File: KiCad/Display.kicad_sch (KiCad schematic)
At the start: 30 parts, among them J1 DC, J2 USB-C, M1 OLED1.5-RGB, U1 L86-M33, U2 ESP32-PICO-MINI-02, U3 FT231XQ, U4 LMR16006+FB, U5 QR

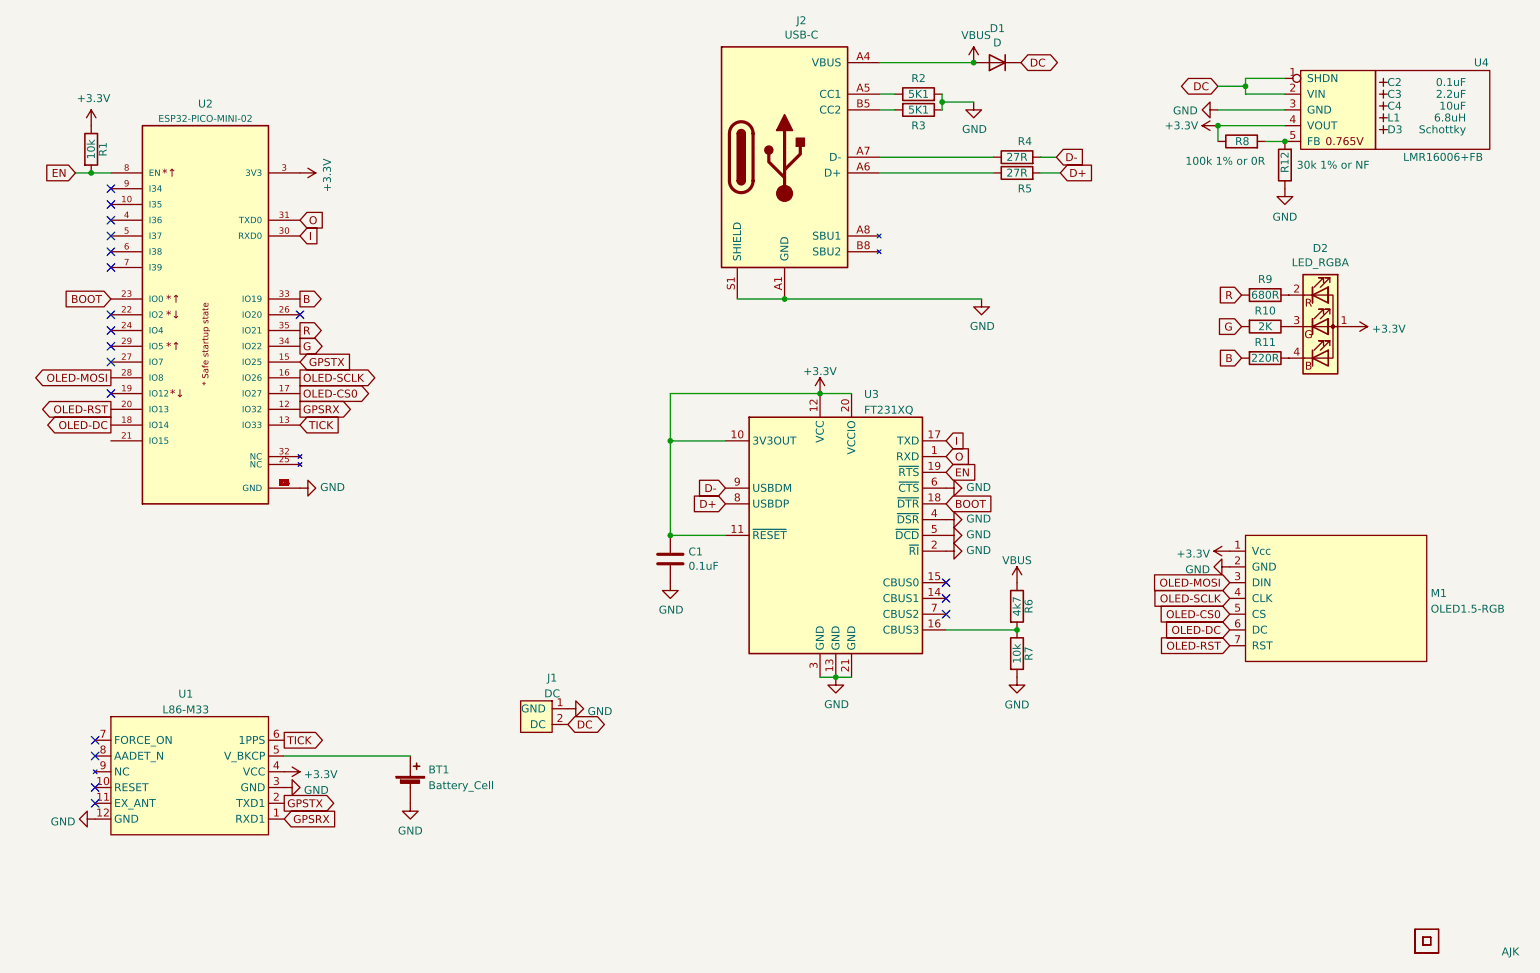
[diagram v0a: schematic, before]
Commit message: Pin names
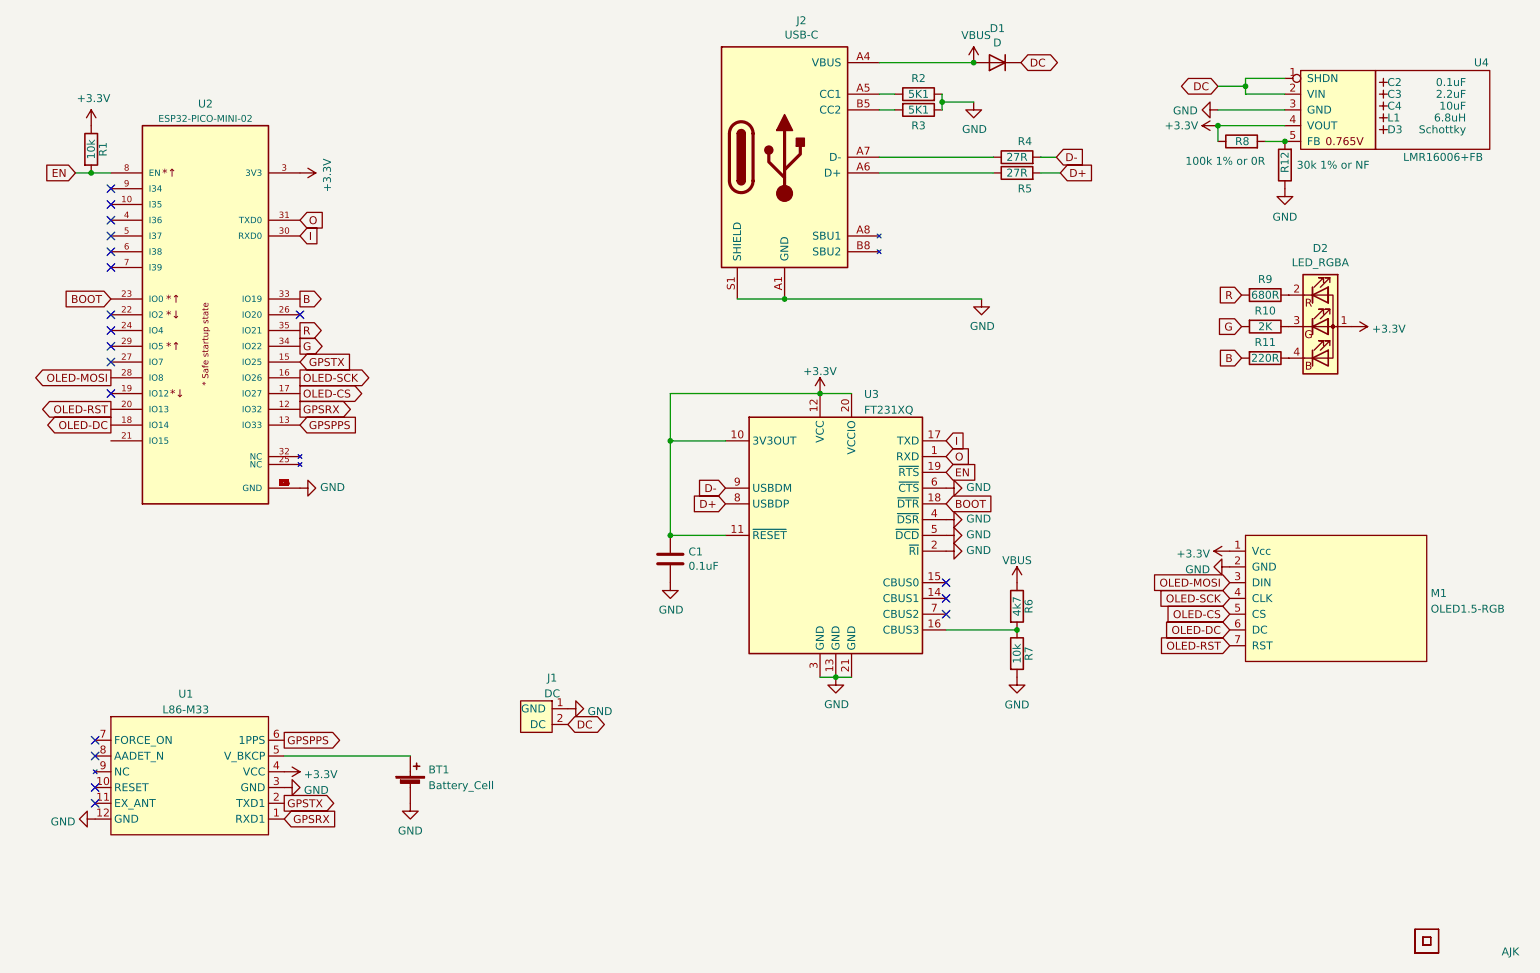
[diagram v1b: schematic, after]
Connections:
- net OLED-CS0 renamed OLED-CS
- net OLED-SCLK renamed OLED-SCK
- net TICK renamed GPSPPS
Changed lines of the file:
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@@
     )
   )
-  (global_label "OLED-SCLK" (shape input) (at 231.14 116.84 180) (fields_autoplaced)
+  (global_label "OLED-SCK" (shape input) (at 231.14 116.84 180) (fields_autoplaced)
     (effects (font (size 1.27 1.27)) (justify right))
-    (property "Intersheet References" "${INTERSHEET_REFS}" (id 0) (at 121.285 -13.335 0)
-      (effects (font (size 1.27 1.27)) hide)
+    (property "Intersheet References" "${INTERSHEET_REFS}" (id 0) (at 218.7163 116.7606 0)
+      (effects (font (size 1.27 1.27)) (justify right) hide)
     )
   )
@@
     )
   )
-  (global_label "OLED-CS0" (shape input) (at 231.14 119.38 180) (fields_autoplaced)
+  (global_label "OLED-CS" (shape input) (at 231.14 119.38 180) (fields_autoplaced)
     (effects (font (size 1.27 1.27)) (justify right))
-    (property "Intersheet References" "${INTERSHEET_REFS}" (id 0) (at 121.285 -13.335 0)
-      (effects (font (size 1.27 1.27)) hide)
+    (property "Intersheet References" "${INTERSHEET_REFS}" (id 0) (at 219.9863 119.3006 0)
+      (effects (font (size 1.27 1.27)) (justify right) hide)
     )
   )
@@
     )
   )
-  (global_label "OLED-CS0" (shape output) (at 81.28 83.82 0) (fields_autoplaced)
+  (global_label "OLED-CS" (shape output) (at 81.28 83.82 0) (fields_autoplaced)
     (effects (font (size 1.27 1.27)) (justify left))
-    (property "Intersheet References" "${INTERSHEET_REFS}" (id 0) (at 93.6432 83.8994 0)
+    (property "Intersheet References" "${INTERSHEET_REFS}" (id 0) (at 92.4337 83.7406 0)
       (effects (font (size 1.27 1.27)) (justify left) hide)
     )
@@
     )
   )
-  (global_label "OLED-SCLK" (shape output) (at 81.28 81.28 0) (fields_autoplaced)
+  (global_label "OLED-SCK" (shape output) (at 81.28 81.28 0) (fields_autoplaced)
     (effects (font (size 1.27 1.27)) (justify left))
-    (property "Intersheet References" "${INTERSHEET_REFS}" (id 0) (at 94.7318 81.2006 0)
+    (property "Intersheet References" "${INTERSHEET_REFS}" (id 0) (at 93.7037 81.2006 0)
       (effects (font (size 1.27 1.27)) (justify left) hide)
     )
@@
     )
   )
-  (global_label "TICK" (shape input) (at 81.28 88.9 0) (fields_autoplaced)
+  (global_label "GPSPPS" (shape input) (at 81.28 88.9 0) (fields_autoplaced)
     (effects (font (size 1.27 1.27)) (justify left))
-    (property "Intersheet References" "${INTERSHEET_REFS}" (id 0) (at 87.7166 88.9794 0)
+    (property "Intersheet References" "${INTERSHEET_REFS}" (id 0) (at 91.1032 88.8206 0)
       (effects (font (size 1.27 1.27)) (justify left) hide)
     )
@@
     )
   )
-  (global_label "TICK" (shape output) (at 78.74 139.7 0) (fields_autoplaced)
+  (global_label "GPSPPS" (shape output) (at 78.74 139.7 0) (fields_autoplaced)
     (effects (font (size 1.27 1.27)) (justify left))
-    (property "Intersheet References" "${INTERSHEET_REFS}" (id 0) (at 85.1766 139.6206 0)
+    (property "Intersheet References" "${INTERSHEET_REFS}" (id 0) (at 88.5632 139.6206 0)
       (effects (font (size 1.27 1.27)) (justify left) hide)
     )
